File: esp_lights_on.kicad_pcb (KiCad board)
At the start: 2 copper layers, 50.7 x 58.5 mm, 14 parts, among them J1 Conn_01x04_Pin, J2 VOUT, J3 VIN, K1 RELAY, Q1 SS8050, U1 ESP32-WROOM-32, U2 TLV1117-33

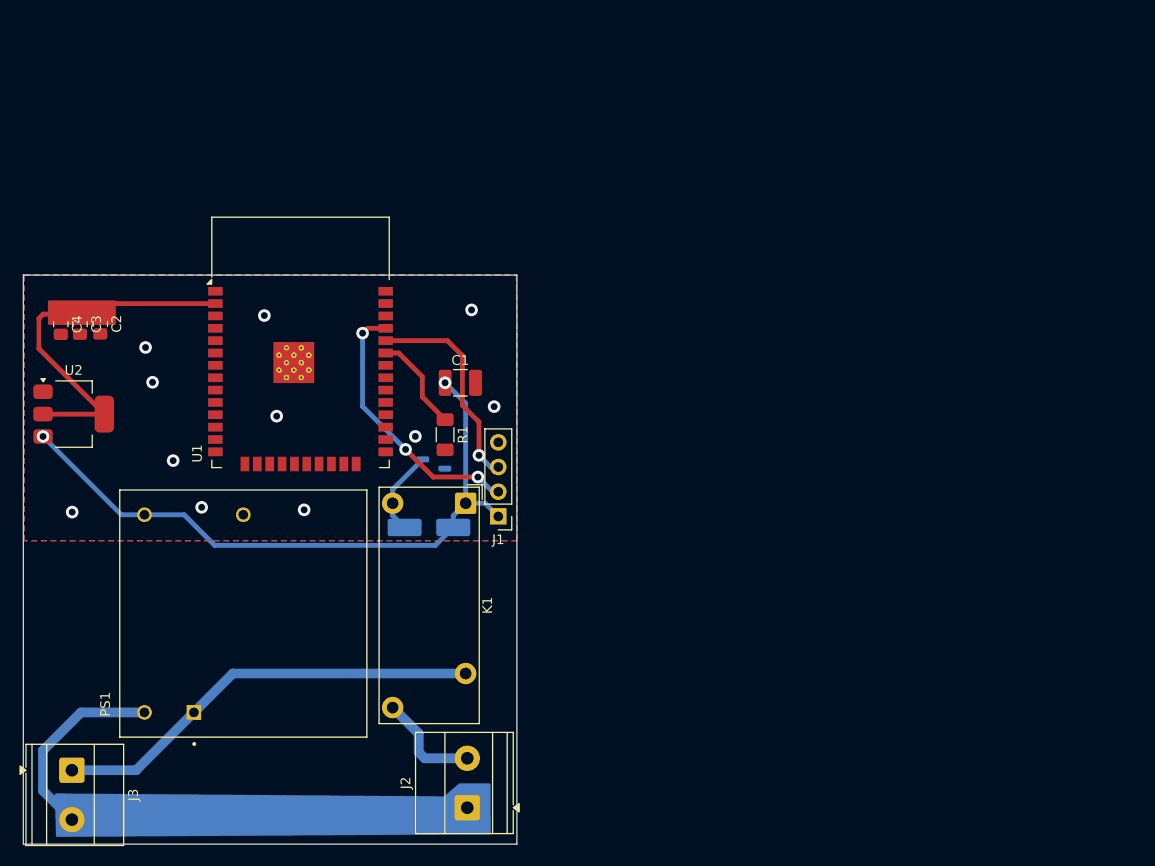
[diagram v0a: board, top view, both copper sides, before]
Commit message: some other updates unverified
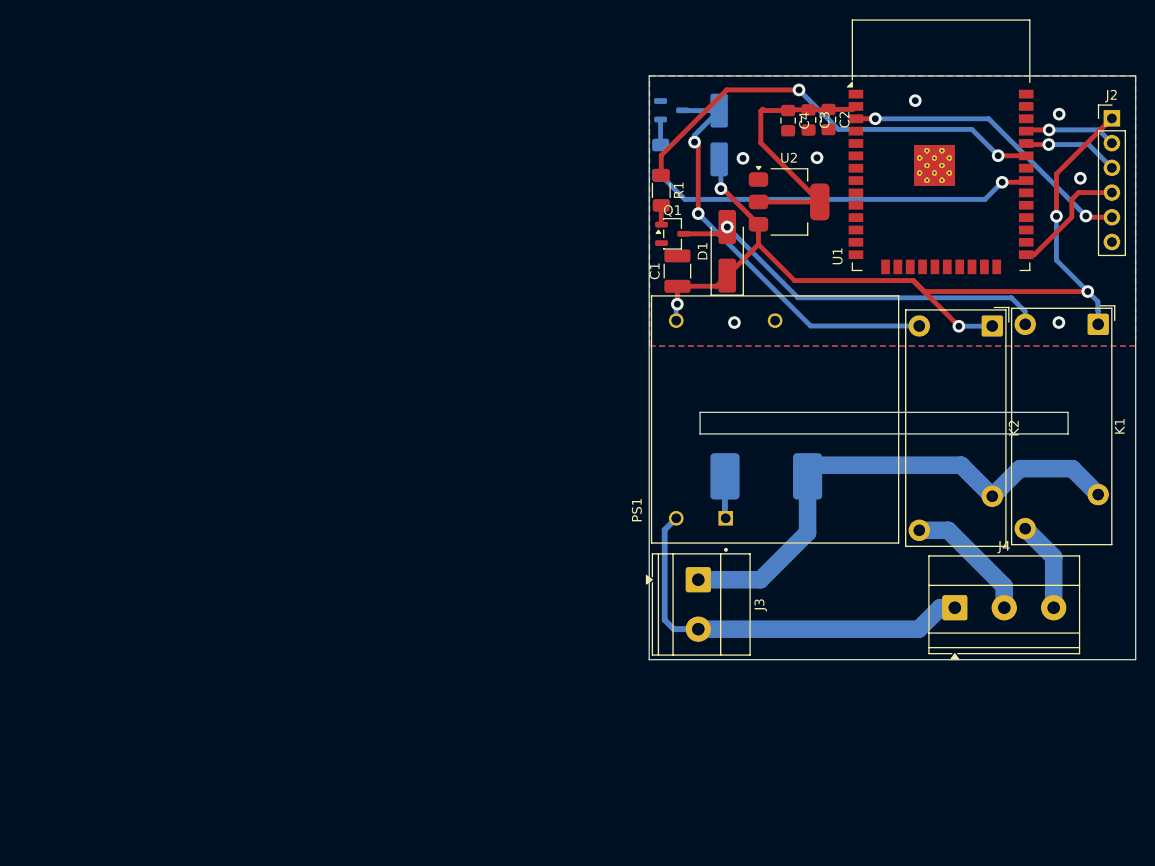
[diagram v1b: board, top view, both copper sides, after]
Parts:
- removed J1: Conn_01x04_Pin, Connector_PinHeader_2.54mm:PinHeader_1x04_P2.54mm_Vertical
- added D2: D, Diode_SMD:D_SMA_Handsoldering, B.Cu at (196.9, 37.3)
- added F1: Fuse_Small, Fuse:Fuse_Schurter_UMZ250, B.Cu at (201.8, 72.4)
- added J4: Screw_Terminal_01x03, TerminalBlock_Phoenix:TerminalBlock_Phoenix_MKDS-1,5-3-5.08_1x03_P5.08mm_Horizontal, F.Cu at (221.1, 85.9)
- added K2: RELAY, Relay_THT:Relay_SPST_Panasonic_ADW11, F.Cu at (225.0, 57.0)
- added Q2: SS8050, Package_TO_SOT_SMD:SOT-23-3, B.Cu at (192.0, 34.8)
- added R2: 1k, Resistor_SMD:R_1206_3216Metric_Pad1.30x1.75mm_HandSolder, B.Cu at (190.9, 39.9)
- D1, Q1: moved to F.Cu
- J2: value VOUT -> Conn_01x06_Pin; footprint TerminalBlock_Phoenix:TerminalBlock_Phoenix_MKDS-1,5-2-5.08_1x02_P5.08mm_Horizontal -> Connector_PinHeader_2.54mm:PinHeader_1x06_P2.54mm_Vertical
- moved J2 97.0 mm to (237.3, 35.6), turned to 0 degrees
- moved C3 77.8 mm to (206.1, 35.8)
- moved C2 77.7 mm to (208.2, 35.7)
- moved C4 77.6 mm to (204.0, 35.8)
- moved U2 76.7 mm to (204.1, 44.2)
- moved U1 68.9 mm to (219.7, 41.4)
- moved K1 67.6 mm to (235.9, 56.8)
- moved J3 67.3 mm to (194.8, 83.0)
- moved PS1 58.2 mm to (202.7, 66.6)
- moved D1 41.8 mm to (197.8, 49.3), turned to 90 degrees
- moved Q1 33.8 mm to (192.1, 47.5), turned to 0 degrees
- moved R1 33.5 mm to (191.0, 43.0)
- moved C1 25.1 mm to (192.6, 51.3), turned to 90 degrees
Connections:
- net COLECTOR renamed COLECTOR1
- net SW renamed SW1
- J2 pad 1: VIN_NULL -> VOUT_5V
- J2 pad 2: VOUT_220V -> RX
- J3 pad 2: VIN_NULL -> NULL
- K1 pad 14: VOUT_220V -> circuit1
- PS1 pad 1: VIN_220V -> VIN_220V_traf
- PS1 pad 2: VIN_NULL -> NULL
- U1 pad 25: unconnected-(U1-IO0-Pad25) -> BOOt
- U1 pad 3: unconnected-(U1-EN-Pad3) -> EN
- U1 pad 31: unconnected-(U1-IO19-Pad31) -> SW2
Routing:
- net COLECTOR2: track 0.00 -> 43.1 mm, vias 0 -> 2
- net NULL: track 0.00 -> 42.1 mm
- net SW2: track 0.00 -> 39.4 mm, vias 0 -> 1
- net SW1: track 10.2 -> 45.1 mm, vias 0 -> 2
- net COLECTOR1: track 8.79 -> 40.3 mm, vias 0 -> 1
- net EN: track 0.00 -> 30.5 mm, vias 0 -> 2
- net VOUT_5V: track 67.8 -> 95.5 mm, vias 2 -> 5
- net VIN_NULL: track 20.4 -> 0.00 mm
- net RX: track 27.7 -> 9.42 mm, vias 3 -> 1
- net circuit2: track 0.00 -> 13.3 mm
- net BOOt: track 0.00 -> 12.5 mm
- net TX: track 22.0 -> 9.85 mm
- net VOUT_220V: track 11.0 -> 0.00 mm
- net circuit1: track 0.00 -> 9.34 mm
- net VIN_220V: track 44.6 -> 53.0 mm
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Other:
- board size 50.7 x 58.5 mm -> 50 x 60 mm
